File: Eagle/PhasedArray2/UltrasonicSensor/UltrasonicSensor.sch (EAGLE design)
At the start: 34 parts

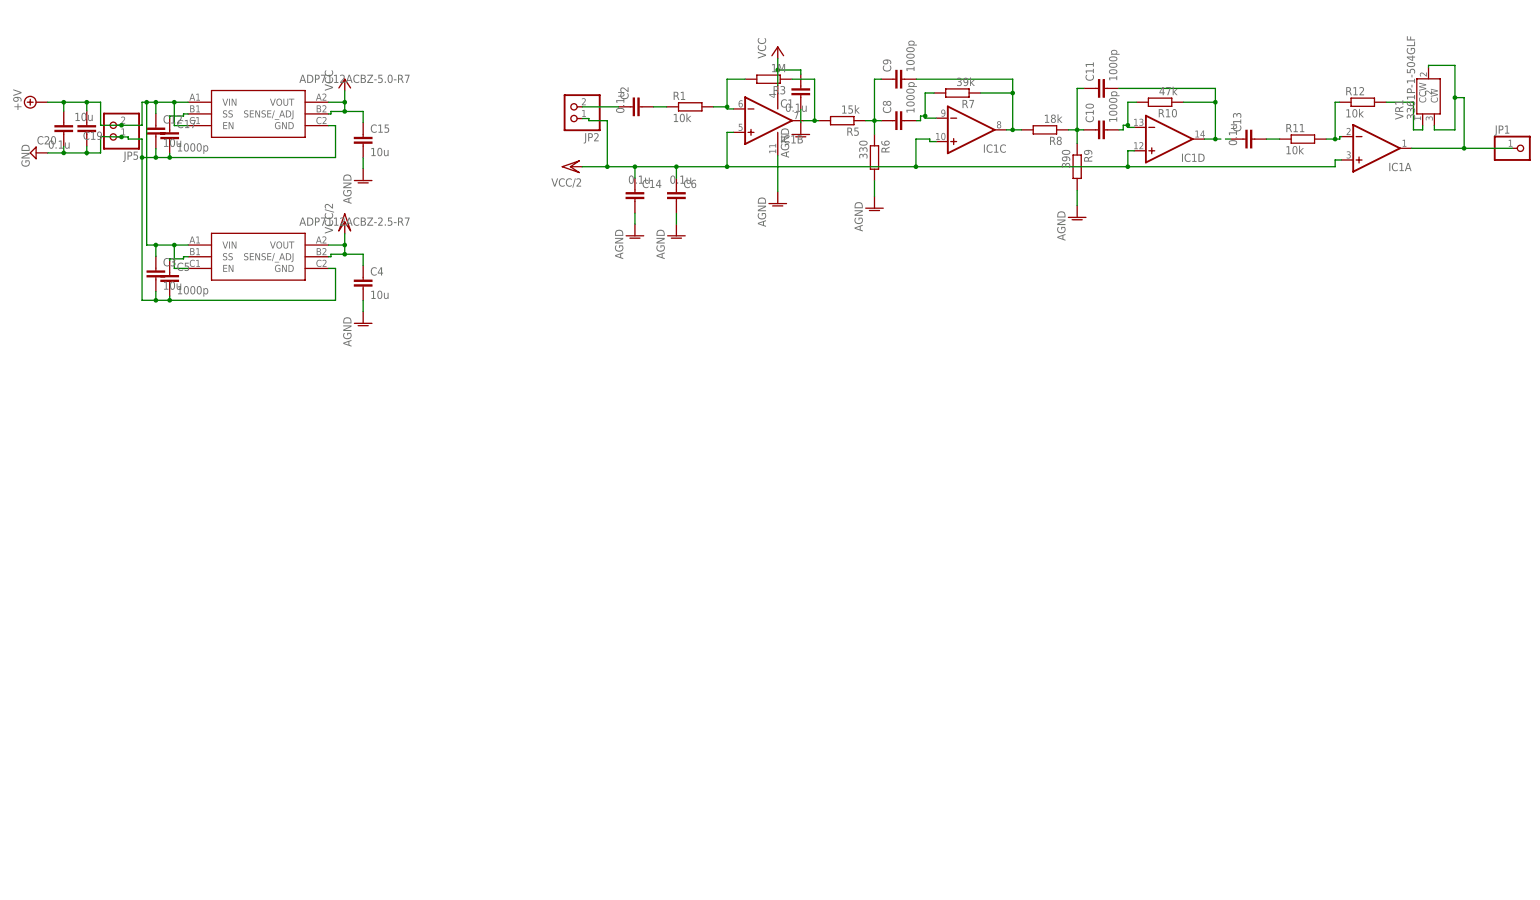
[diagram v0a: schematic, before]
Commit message: Add files via upload
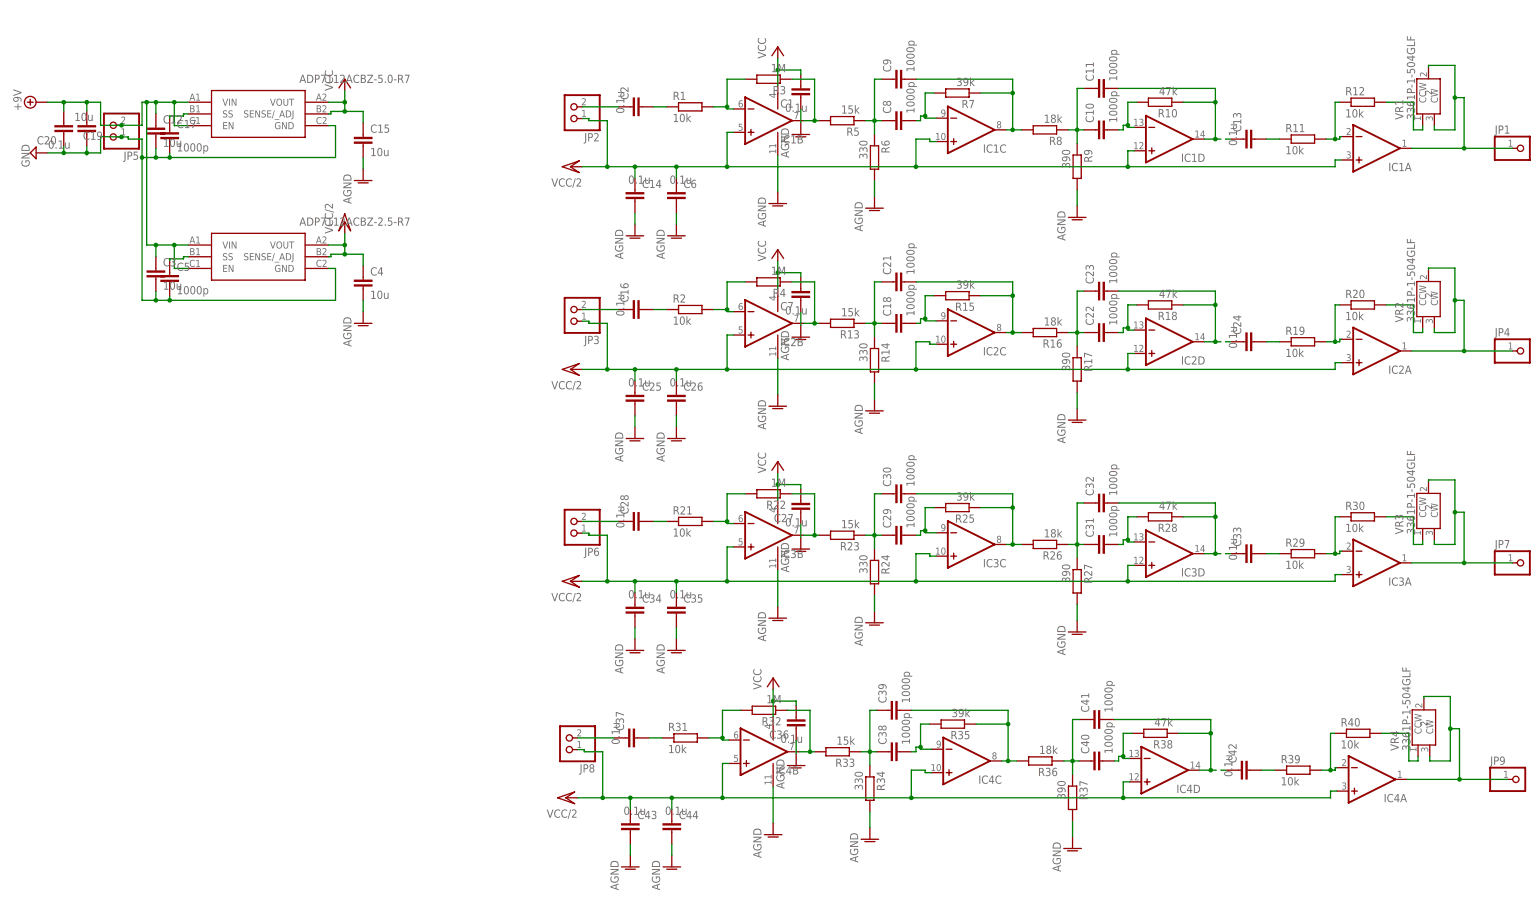
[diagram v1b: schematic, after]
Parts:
- added C16, C24, C25, C26, C27, C28, C33, C34, C35, C36, C37, C42, C43, C44, C7: 0.1u, rcl:C-EUC1608
- added C18, C21, C22, C23, C29, C30, C31, C32, C38, C39, C40, C41: 1000p, rcl:C-EUC1608
- added IC2, IC3, IC4: (no value), linear3:NJM2734M
- added JP3, JP6, JP8: (no value), pinhead:PINHD-1X2
- added JP4, JP7, JP9: (no value), pinhead:PINHD-1X1
- added R13, R23, R33: 15k, rcl:R-EU_R0603
- added R14, R24, R34: 330, rcl:R-EU_R0603
- added R15, R25, R35: 39k, rcl:R-EU_R0603
- added R16, R26, R36: 18k, rcl:R-EU_R0603
- added R17, R27, R37: 390, rcl:R-EU_R0603
- added R18, R28, R38: 47k, rcl:R-EU_R0603
- added R19, R2, R20, R21, R29, R30, R31, R39, R40: 10k, rcl:R-EU_R0603
- added R22, R32, R4: 1M, rcl:R-EU_R0603
- added VR2, VR3, VR4: 3361P-1-504GLF, 3361P-1-504GLF:3361P-1-504GLF
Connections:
- new net N$1: C16.2, R2.1
- new net N$17: C16.1, JP3.2
- new net N$18: IC2B.OUT, R13.2, R4.1
- new net N$19: C18.1, C21.1, R13.1, R14.1
- new net N$20: IC2B.-IN, R2.2, R4.2
- new net N$21: C18.2, IC2C.-IN, R15.2
- new net N$22: C21.2, IC2C.OUT, R15.1, R16.2
- new net N$23: C22.1, C23.1, R16.1, R17.1
- new net N$24: C22.2, IC2D.-IN, R18.2
- new net N$25: C23.2, C24.1, IC2D.OUT, R18.1
- new net N$26: C24.2, R19.1
- new net N$27: IC2A.-IN, R19.2, R20.1
- new net N$28: R20.2, VR2.CCW
- new net N$29: IC2A.OUT, JP4.1, VR2.2, VR2.CW
- new net N$30: C28.2, R21.1
- new net N$31: C28.1, JP6.2
- new net N$32: IC3B.OUT, R22.1, R23.2
- new net N$33: C29.1, C30.1, R23.1, R24.1
- new net N$35: IC3B.-IN, R21.2, R22.2
- new net N$36: C29.2, IC3C.-IN, R25.2
- new net N$37: C30.2, IC3C.OUT, R25.1, R26.2
- new net N$38: C31.1, C32.1, R26.1, R27.1
- new net N$39: C31.2, IC3D.-IN, R28.2
- new net N$40: C32.2, C33.1, IC3D.OUT, R28.1
- new net N$41: C33.2, R29.1
- new net N$42: IC3A.-IN, R29.2, R30.1
- new net N$43: R30.2, VR3.CCW
- new net N$44: IC3A.OUT, JP7.1, VR3.2, VR3.CW
- new net N$45: C37.2, R31.1
- new net N$46: C37.1, JP8.2
- new net N$47: IC4B.OUT, R32.1, R33.2
- new net N$48: C38.1, C39.1, R33.1, R34.1
- new net N$49: IC4B.-IN, R31.2, R32.2
- new net N$50: C38.2, IC4C.-IN, R35.2
- new net N$51: C39.2, IC4C.OUT, R35.1, R36.2
- new net N$52: C40.1, C41.1, R36.1, R37.1
- new net N$53: C40.2, IC4D.-IN, R38.2
- new net N$54: C41.2, C42.1, IC4D.OUT, R38.1
- new net N$55: C42.2, R39.1
- new net N$56: IC4A.-IN, R39.2, R40.1
- new net N$57: R40.2, VR4.CCW
- new net N$58: IC4A.OUT, JP9.1, VR4.2, VR4.CW
- net AGND: now also C25.2, C26.2, C27.1, C34.2, C35.2, C36.1, C43.2, C44.2, C7.1, IC2P.V-, IC3P.V-, IC4P.V-, R14.2, R17.2, R24.2, R27.2, R34.2, R37.2
- net VCC: now also C27.2, C36.2, C7.2, IC2P.V+, IC3P.V+, IC4P.V+
- net VCC/2: now also C25.1, C26.1, C34.1, C35.1, C43.1, C44.1, IC2A.+IN, IC2B.+IN, IC2C.+IN, IC2D.+IN, IC3A.+IN, IC3B.+IN, IC3C.+IN, IC3D.+IN, IC4A.+IN, IC4B.+IN, IC4C.+IN, IC4D.+IN, JP3.1, JP6.1, JP8.1
